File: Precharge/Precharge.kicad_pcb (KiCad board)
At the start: 2 copper layers, 87.1 x 86.1 mm, 62 parts, among them J1 Conn_01x02, J2 Conn_01x02, J3 Molex MicroFit, J4 Conn_02x03_Counter_Clockwise, K1 KT12-1A-40L-THT, Q1 AO3400A, Q2 2N7002, U1 LM393, U2 4N35, U3 4N35, U4 NE555D

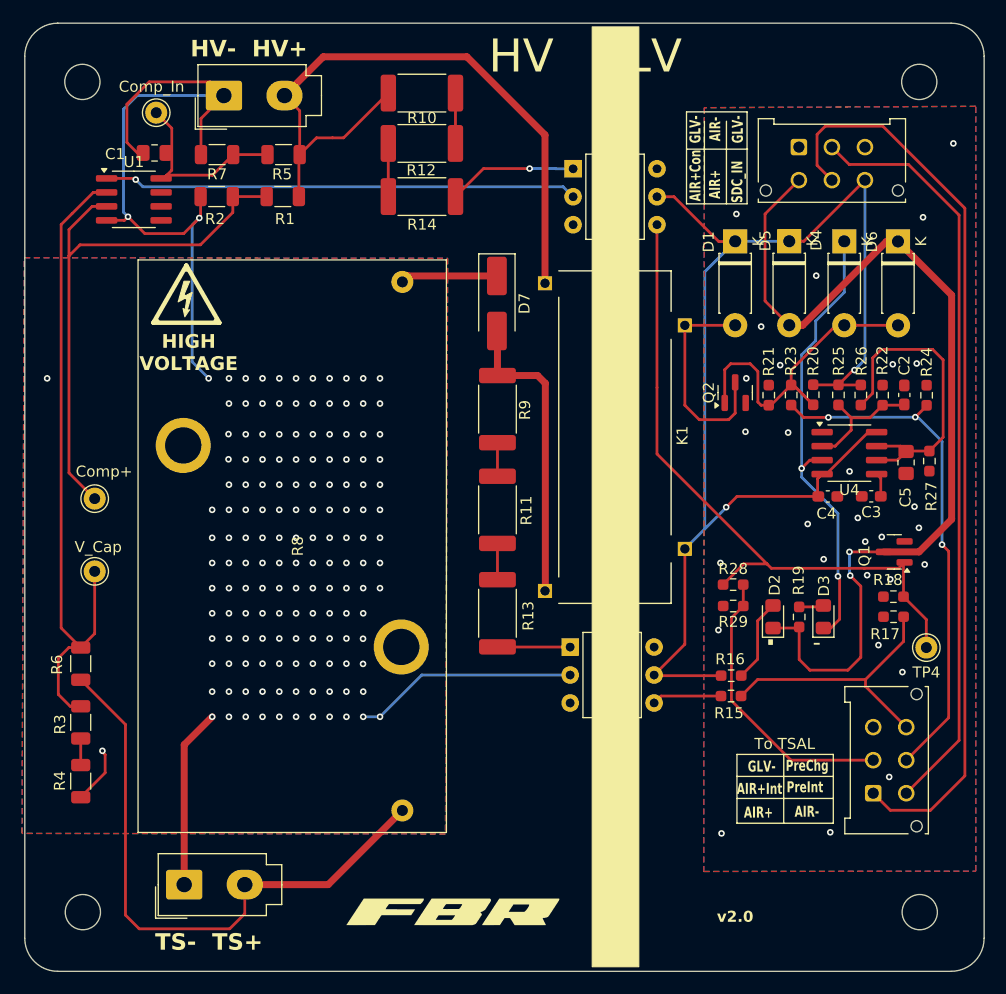
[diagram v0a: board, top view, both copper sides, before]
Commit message: v2.1
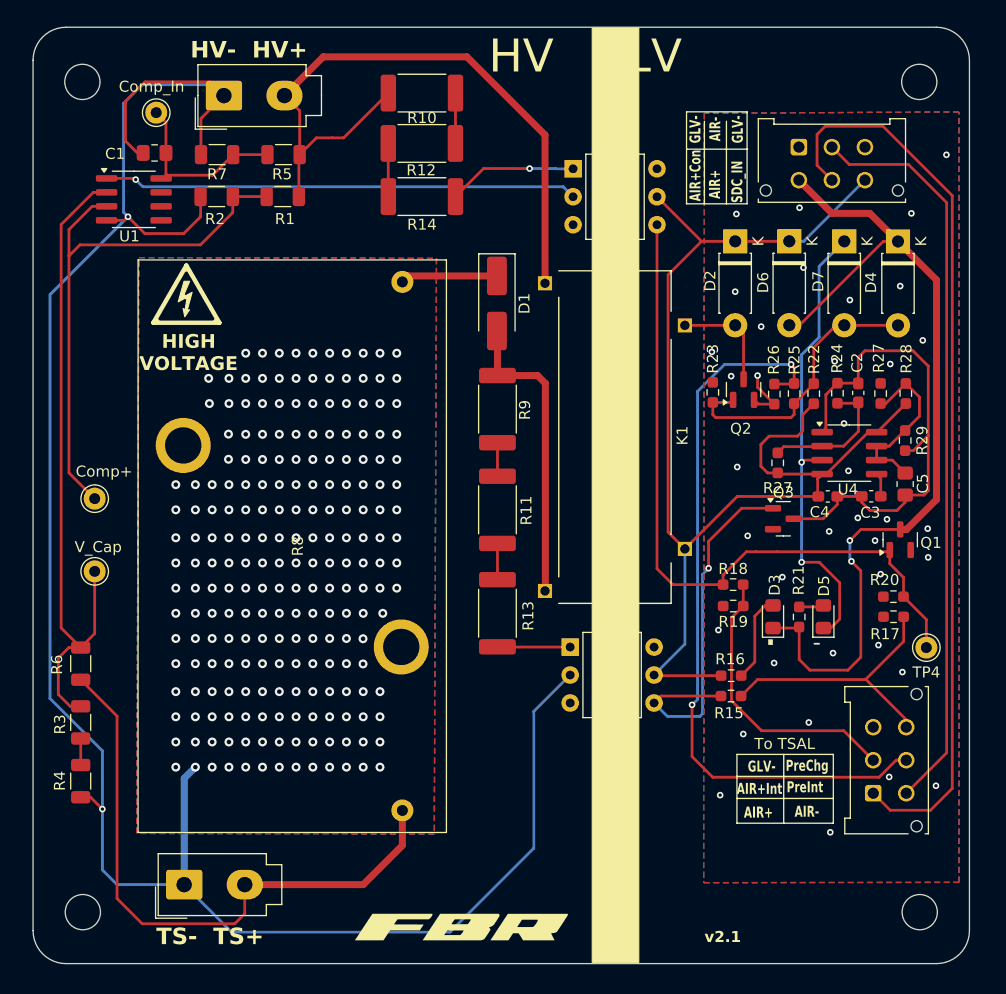
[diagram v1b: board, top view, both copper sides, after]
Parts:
- added Q3: 2N7002, Package_TO_SOT_SMD:SOT-23, F.Cu at (139.0, 96.3)
- added R29: 1M, Resistor_SMD:R_0603_1608Metric_Pad0.98x0.95mm_HandSolder, F.Cu at (150.1, 89.2)
- R8: value 120 -> 150
- moved R26 13.8 mm to (138.2, 85.0), turned to -90 degrees
- moved R27 8.28 mm to (138.5, 91.2), turned to 90 degrees
- moved R27 7.57 mm to (147.8, 84.9), turned to 90 degrees
- moved R23 5.09 mm to (132.6, 84.8)
- moved C2 4.18 mm to (145.8, 84.9)
- moved R24 4.10 mm to (143.9, 84.9)
- moved R28 4.09 mm to (150.1, 84.9), turned to 90 degrees
- moved C5 1.96 mm to (150.1, 93.2)
- moved G*** 1.59 mm to (109.6, 133.3)
- moved Q1 1.23 mm to (149.6, 98.2), turned to 90 degrees
- moved Q2 0.81 mm to (135.4, 84.6)
- moved R25 0.30 mm to (140.0, 84.9), turned to 90 degrees
- moved R22 0.11 mm to (141.8, 85.0), turned to -90 degrees
- renumbered D7 to D1, D1 to D2, D2 to D3, D6 to D4, D3 to D5, D5 to D6, D4 to D7, R28 to R18, R29 to R19, R18 to R20, R19 to R21, R20 to R22, R21 to R23, R22 to R24, R23 to R25, R24 to R26, R25 to R27, R26 to R28
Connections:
- net Net-(R15-Pad2) renamed /Precharge_12V
- C2 pad 2: GLV- -> Net-(Q3-D)
- C3 pad 2: GLV- -> Net-(Q3-D)
- C4 pad 2: GLV- -> Net-(Q3-D)
- C5 pad 2: GLV- -> Net-(Q3-D)
- R24 pad 1: GLV- -> Net-(Q3-D)
- U1 pad 5: unconnected-(U1B-+-Pad5) -> (no net)
- U1 pad 6: unconnected-(U1B---Pad6) -> (no net)
- U1 pad 7: unconnected-(U1-Pad7) -> (no net)
- U4 pad 1: GLV- -> Net-(Q3-D)
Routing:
- net HV-: track 110.8 -> 194.4 mm, vias 150 -> 217
- net Net-(Q3-D): track 0.00 -> 45.9 mm
- net /Precharge_12V: track 6.34 -> 34.3 mm, vias 0 -> 1
- net /PreCh_Int: track 47.4 -> 67.4 mm, vias 3 -> 2
- net Net-(U4-DIS): track 28.6 -> 15.9 mm
- net Net-(D2-A): track 20.0 -> 9.80 mm
- net /AIR+_Con: track 87.9 -> 81.7 mm
- net Net-(D4-A): track 31.7 -> 26.3 mm
- net GLV-: track 0.26 -> 5.23 mm, vias 29 -> 38
- net /PreCh_Complt: track 61.3 -> 65.1 mm
- net /SDC_IN: track 116.0 -> 113.1 mm, vias 2 -> 0
- net Net-(U4-TR): track 11.3 -> 12.7 mm
- net Net-(U1C-V+): track 17.2 -> 16.0 mm
- net Net-(J2-Pin_2): track 54.7 -> 55.8 mm
- net /AIR+: track 83.3 -> 82.4 mm
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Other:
- board size 87.1 x 86.1 mm -> 85 x 85 mm
- board text added: "0.2000 mm / 0.2000 mm"
- board text added: "0.3000 mm"
- board text added: "1.6000 mm"
- board text added: "2"
- board text added: "85.0372 mm x 85.0344 mm"
- board text added: "BOARD CHARACTERISTICS"
- board text added: "Board Thickness:"
- board text added: "Board overall dimensions:"
- board text added: "Castellated pads:"
- board text added: "Copper Finish:"
- board text added: "Copper Layer Count:"
- board text added: "Edge card connectors:"
- board text added: "Impedance Control:"
- board text added: "Min hole diameter:"
- board text added: "Min track/spacing:"
- board text added: "No"
- board text added: "None"
- board text added: "Plated Board Edge:"
- board text added: "v2.1"
- board text removed: "v2.0"
